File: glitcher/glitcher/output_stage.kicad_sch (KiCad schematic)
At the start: 26 parts, among them J3 Conn_01x03, J4 Conn_01x03, J5 Conn_01x03, J6 Conn_01x03, J7 Conn_01x03, U3 max4619cpe+, U9_3V3ALWAYS1 LD1117S33TR_SOT223

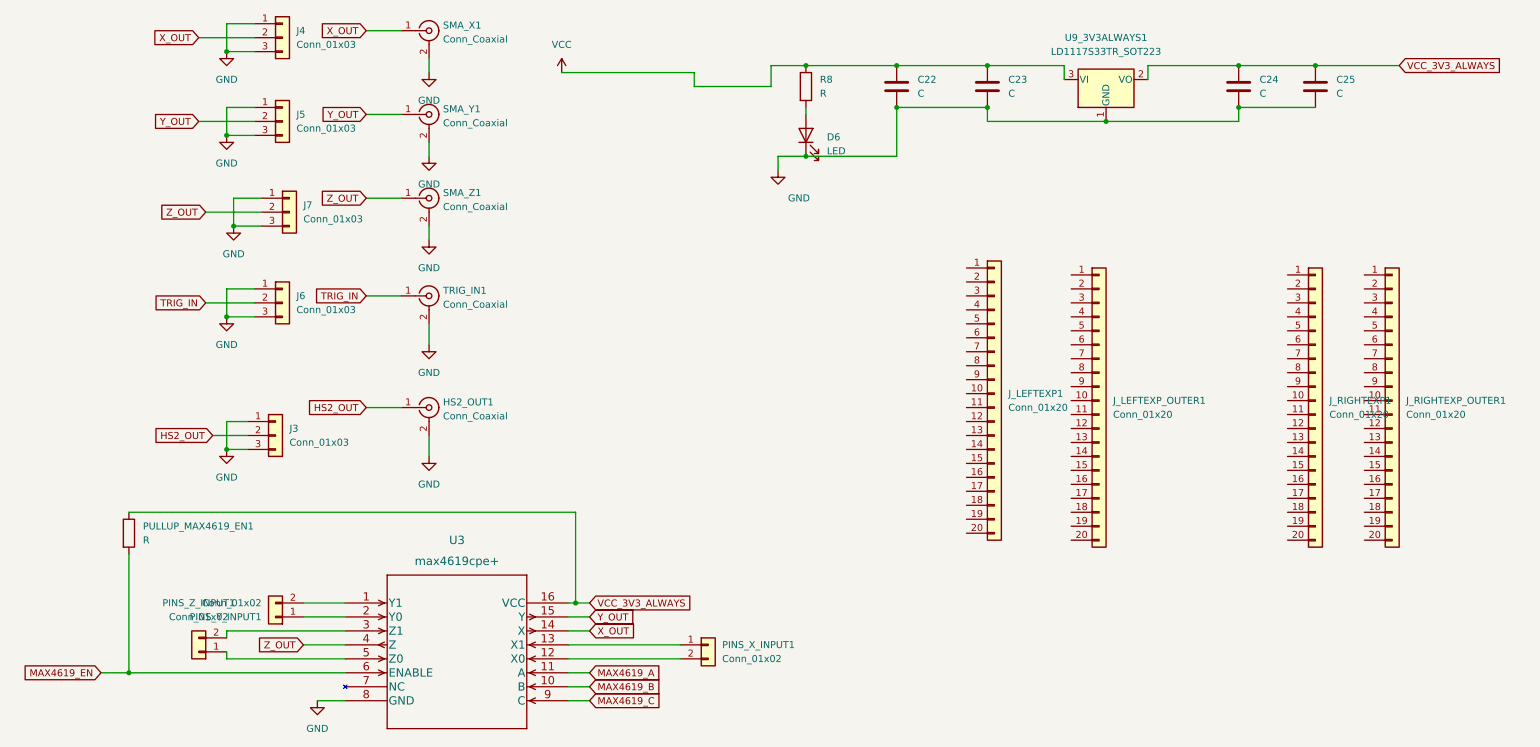
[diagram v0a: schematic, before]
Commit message: lolsave
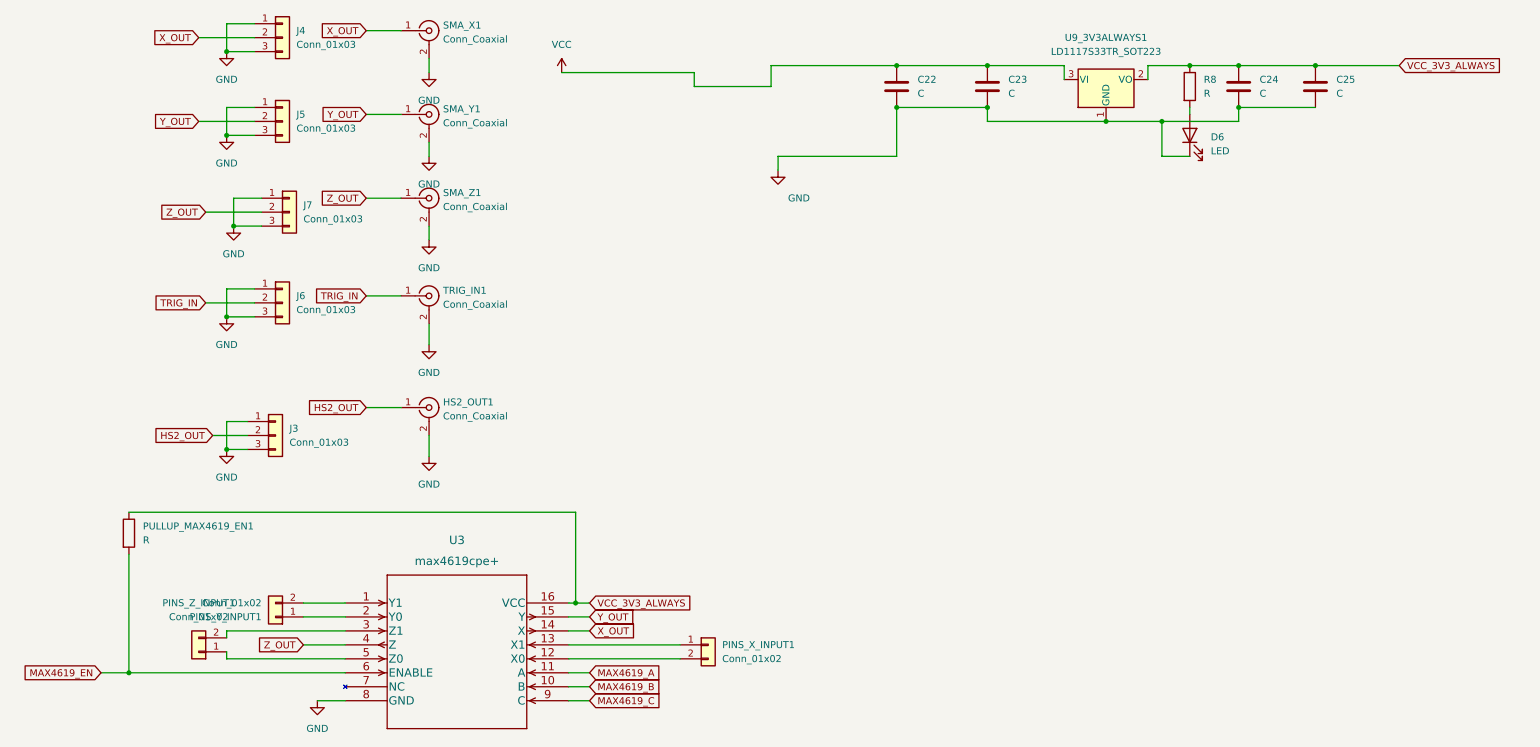
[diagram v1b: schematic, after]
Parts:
- removed J_LEFTEXP1, J_LEFTEXP_OUTER1, J_RIGHTEXP1, J_RIGHTEXP_OUTER1: Conn_01x20, Connector_PinHeader_2.54mm:PinHeader_1x20_P2.54mm_Vertical, symbol Connector_Generic:Conn_01x20
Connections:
- net VCC: no longer R8.1
- net VCC_3V3_ALWAYS: now also R8.1
